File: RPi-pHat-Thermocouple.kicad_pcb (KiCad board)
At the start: 2 copper layers, 65 x 30 mm, 47 parts, among them J1 Screw_Terminal_01x02, J2 RPi_GPIO, J3 Screw_Terminal_01x02, J4 Screw_Terminal_01x02, J5 Screw_Terminal_01x02, J6 Screw_Terminal_01x03, J7 Screw_Terminal_01x04, U1 MCP1754ST, U2 DS18S20, U3 MAX31850K, U4 MAX31850K, U5 MAX31850K, U6 MAX3221CDBR, U7 ADuM1201ARZ

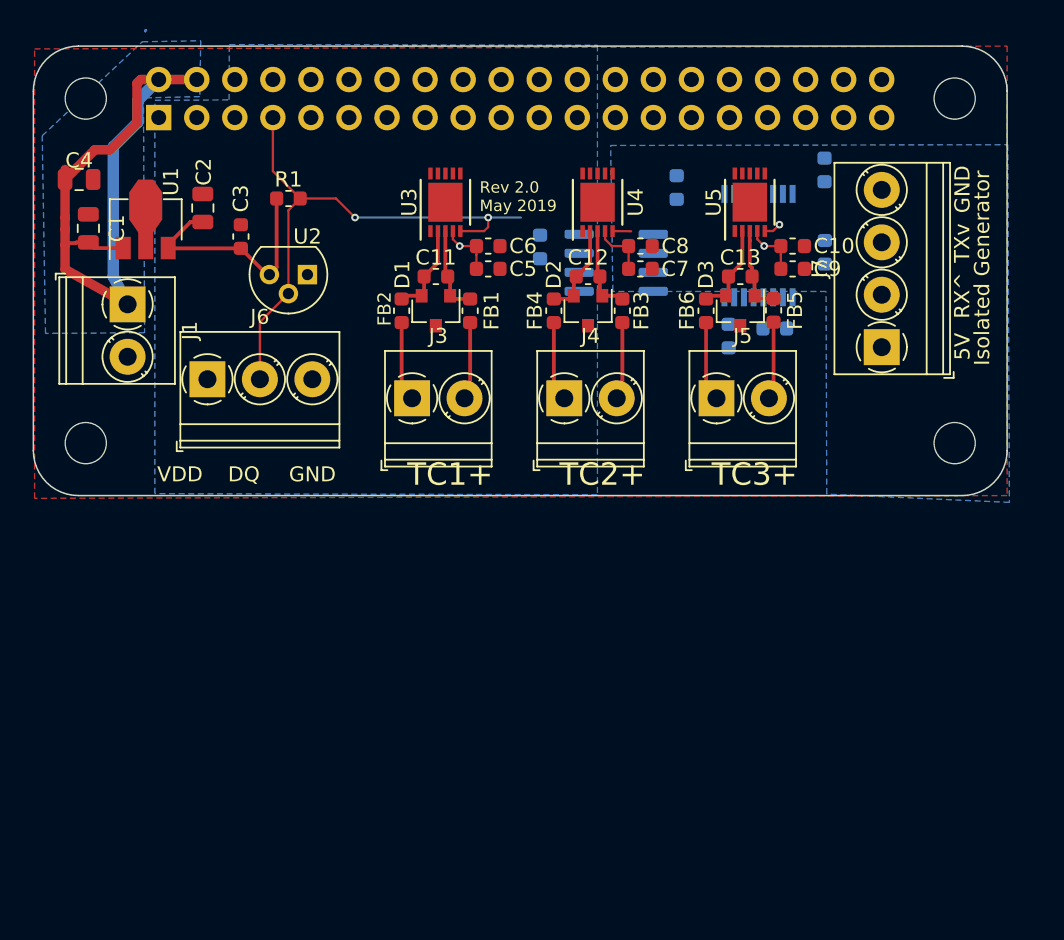
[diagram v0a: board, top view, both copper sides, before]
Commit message: PCB Version 3.0 files
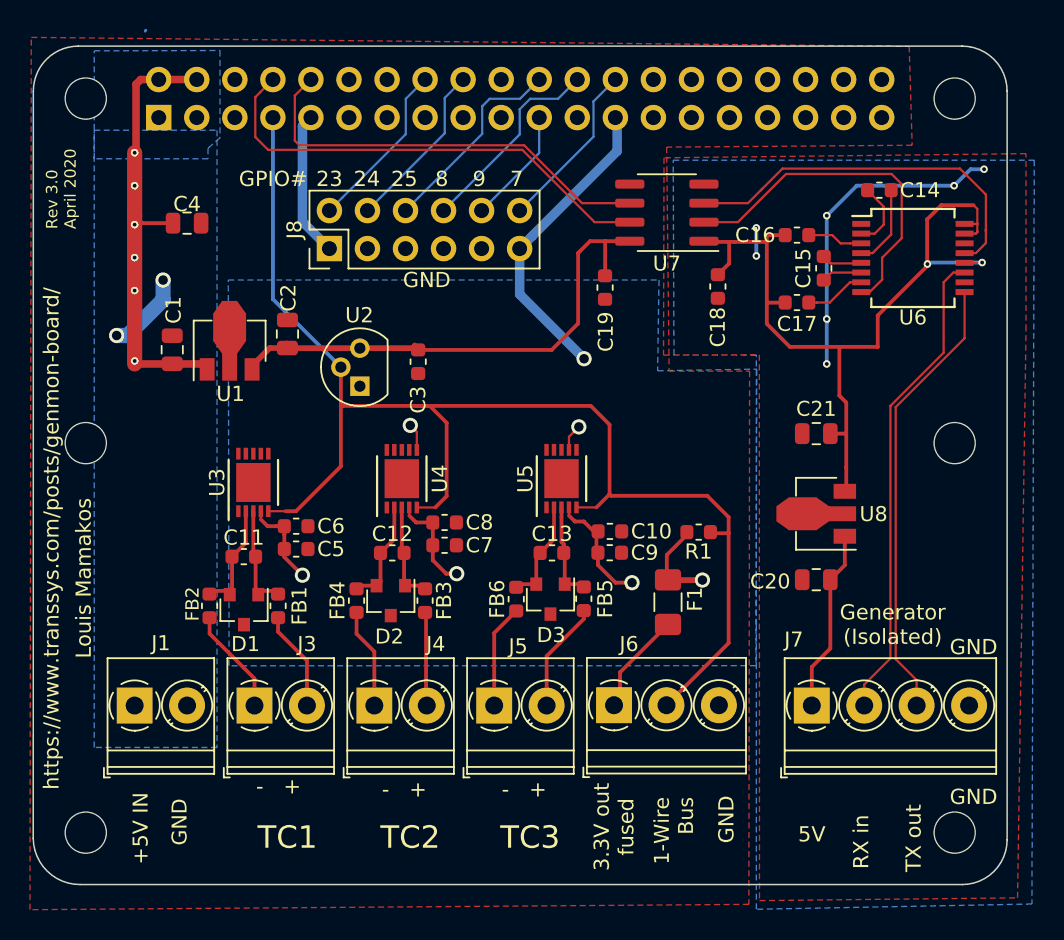
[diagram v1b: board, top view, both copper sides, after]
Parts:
- added C20: 2.2uF, Capacitor_SMD:C_0805_2012Metric, F.Cu at (64.8, 60.1)
- added C21: 2.2uF, Capacitor_SMD:C_0805_2012Metric, F.Cu at (64.8, 50.4)
- added F1: Polyfuse 1206L010/60WR 0.1A, Fuse:Fuse_1206_3216Metric_Pad1.42x1.75mm_HandSolder, F.Cu at (54.9, 61.6)
- added J8: Conn_02x06_Odd_Even, Connector_PinHeader_2.54mm:PinHeader_2x06_P2.54mm_Vertical, F.Cu at (32.3, 38.0)
- added U8: MCP1754ST, Package_TO_SOT_SMD:SOT-89-3, F.Cu at (65.2, 55.7)
- added h5: , RPi_Hat:RPi_Hat_Mounting_Hole, F.Cu at (74.0, 77.0)
- added h6: , RPi_Hat:RPi_Hat_Mounting_Hole, F.Cu at (16.0, 77.0)
- C14, C15, C16, C17, C18, C19, U6: moved to F.Cu
- U3: value MAX31850K -> MAX31850KATB
- U4, U5: value MAX31850K -> MAX31850KATB+T
- U7: value ADuM1201ARZ -> ADuM1201ARZ-RL7; moved to F.Cu
- moved R1 35.3 mm to (56.9, 56.9)
- moved J6 34.8 mm to (51.3, 68.5)
- moved J1 26.8 mm to (19.3, 68.5), turned to 0 degrees
- moved J5 25.3 mm to (43.3, 68.5)
- moved J7 24.4 mm to (64.5, 68.5), turned to 0 degrees
- moved J4 24.1 mm to (35.3, 68.5)
- moved D1 23.7 mm to (26.6, 62.1)
- moved FB2 23.5 mm to (24.3, 61.9)
- moved FB1 23.5 mm to (28.8, 61.9)
- moved D2 23.4 mm to (36.4, 61.5)
- moved FB3 23.4 mm to (38.6, 61.5)
- moved FB4 23.4 mm to (34.1, 61.5)
- moved J3 23.1 mm to (27.3, 68.5)
- moved FB5 23.0 mm to (49.2, 61.4)
- moved FB6 23.0 mm to (44.7, 61.4)
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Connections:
- net /GENGND renamed Net-(C18-Pad2)
- C16 pad 2: /GEN5V -> /GEN3V3
- C17 pad 2: /GEN5V -> /GEN3V3
- C18 pad 1: /GEN5V -> /GEN3V3
- J2 pad 16: Net-(J2-Pad16) -> GPIO23
- J2 pad 18: Net-(J2-Pad18) -> GPIO24
- J2 pad 21: Net-(J2-Pad21) -> /GPIO9
- J2 pad 22: Net-(J2-Pad22) -> GPIO25
- J2 pad 24: Net-(J2-Pad24) -> GPIO8
- J2 pad 26: Net-(J2-Pad26) -> GPIO7
- J6 pad 1: +3.3VA -> Net-(F1-Pad1)
- U6 pad 12: /GEN5V -> /GEN3V3
- U6 pad 15: /GEN5V -> /GEN3V3
- U6 pad 16: /GEN5V -> /GEN3V3
- U7 pad 1: /GEN5V -> /GEN3V3
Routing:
- net /GEN3V3: track 0.00 -> 56.1 mm, vias 0 -> 2
- net /W1: track 39.6 -> 91.2 mm, vias 3 -> 0
- net +3.3VA: track 27.7 -> 66.2 mm, vias 2 -> 6
- net GND: track 0.00 -> 35.7 mm, vias 0 -> 3
- net /TXD: track 0.00 -> 31.7 mm
- net /GENIN: track 0.62 -> 32.1 mm
- net /GENOUT: track 0.00 -> 30.1 mm
- net /RXD: track 0.00 -> 29.3 mm
- net Net-(U6-Pad13): track 0.00 -> 25.8 mm
- net Net-(C18-Pad2): track 0.00 -> 23.7 mm, vias 0 -> 7
- net Net-(U6-Pad8): track 0.00 -> 23.5 mm
- net +5V: track 45.2 -> 31.5 mm, vias 0 -> 6
- net GPIO25: track 0.00 -> 13.6 mm
- net GPIO8: track 0.00 -> 13.5 mm
- net /GEN5V: track 0.00 -> 12.2 mm
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- added copper zone on B.Cu, net /GEN5V
- added copper zone on F.Cu, net Net-(C18-Pad2)
- removed copper zone on B.Cu, net Net-(C18-Pad2)
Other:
- board size 65 x 30 mm -> 65 x 56 mm
- board text added: "+ -"
- board text added: "+3.3V"
- board text added: "+5DC to Raspberry Pi"
- board text added: "+5V IN"
- board text added: "- +"
- board text added: "1-Wire Bus"
- board text added: "23"
- board text added: "24"
- board text added: "25"
- board text added: "3.3V out (fused)"
- board text added: "3.3V out fused"
- board text added: "7"
- board text added: "8"
- board text added: "9"
- board text added: "GND TX RX +5 Isolated Generator Controller Signals"
- board text added: "GPIO#"
- board text added: "Generator (Isolated)"
- board text added: "Generator Controller Isolated +5V"
- board text added: "Generator power supply and RS-232 signals isolated from Raspberry Pi and power supply. Do not interconnect generator ground and power supply with Raspberry Pi power to preserve galvanic isolation from controller and avoid ground loops."
- board text added: "Louis Mamakos"
- board text added: "RX in"
- board text added: "Rev 3.0 April 2020"
- board text added: "TX out"
- board text added: "Thermocouple Hat by Louis Mamakos (based on a design by Mike Lawrence)"
- board text added: "Type K Thermocouple Connections"
- board text added: "^ External DS18B20 temperature sensor connection."
- board text added: "https://www.transsys.com/posts/genmon-board/"
- board text removed: "DQ"
- board text removed: "Isolated Generator"
- board text removed: "RX^"
- board text removed: "Rev 2.0 May 2019"
- board text removed: "TC1+"
- board text removed: "TC2+"
- board text removed: "TC3+"
- board text removed: "TXv"
- board text removed: "Thermocouple pHat by Mike Lawrence"
- board text removed: "VDD"

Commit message: Candidate files for Version 3.1 of the PCB
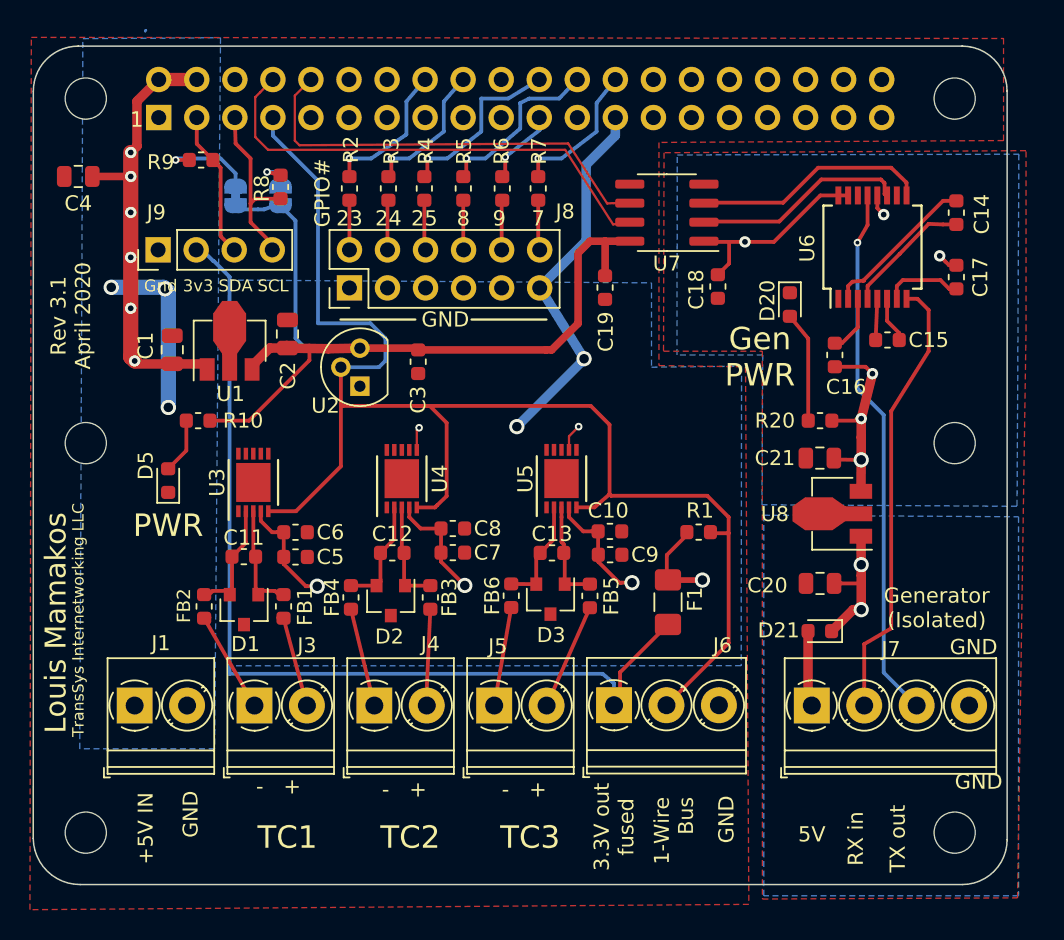
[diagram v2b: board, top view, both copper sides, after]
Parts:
- added D20: ASMT-RF45-AN002, LED_SMD:LED_0603_1608Metric, F.Cu at (63.0, 41.8)
- added D21: NSR20F30NXT5G, Diode_SMD:D_0603_1608Metric, F.Cu at (65.0, 63.5)
- added D5: ASMT-RF45-AN002, LED_SMD:LED_0603_1608Metric, F.Cu at (21.5, 53.5)
- added J9: Conn_01x04_Male, Connector_PinHeader_2.54mm:PinHeader_1x04_P2.54mm_Vertical, F.Cu at (20.8, 38.1)
- added JP1: Jumper_NC_Small, Jumper:SolderJumper-2_P1.3mm_Bridged_RoundedPad1.0x1.5mm, B.Cu at (29.0, 34.5)
- added JP2: Jumper_NC_Small, Jumper:SolderJumper-2_P1.3mm_Bridged_RoundedPad1.0x1.5mm, B.Cu at (26.0, 34.5)
- added R10: 120, Resistor_SMD:R_0603_1608Metric, F.Cu at (23.5, 49.5)
- added R2: 330, Resistor_SMD:R_0603_1608Metric, F.Cu at (33.6, 34.0)
- added R20: 120, Resistor_SMD:R_0603_1608Metric, F.Cu at (65.0, 49.5)
- added R3: 330, Resistor_SMD:R_0603_1608Metric, F.Cu at (36.2, 34.0)
- added R4: 330, Resistor_SMD:R_0603_1608Metric, F.Cu at (38.6, 34.0)
- added R5: 330, Resistor_SMD:R_0603_1608Metric, F.Cu at (41.2, 34.0)
- added R6: 330, Resistor_SMD:R_0603_1608Metric, F.Cu at (43.8, 34.0)
- added R7: 330, Resistor_SMD:R_0603_1608Metric, F.Cu at (46.2, 34.0)
- added R8: 4.7k, Resistor_SMD:R_0603_1608Metric, F.Cu at (29.0, 33.9)
- added R9: 4.7k, Resistor_SMD:R_0603_1608Metric, F.Cu at (23.7, 32.1)
- C14: value 0.047uF -> 0.1uF
- C15, C16, C17: value 0.33uF -> 0.1uF
- U2: value DS18S20 -> DS18B20
- U3: value MAX31850KATB -> MAX31850KATB
- U4, U5: value MAX31850KATB+T -> MAX31850KATB
- U7: value ADuM1201ARZ-RL7 -> ADuM1201AR
- moved C17 10.8 mm to (74.1, 39.9), turned to 90 degrees
- moved C16 8.39 mm to (66.0, 45.1), turned to 270 degrees
- moved C4 7.90 mm to (15.5, 33.2), turned to 180 degrees
- moved C15 6.40 mm to (69.5, 44.1), turned to 0 degrees
- moved C14 5.35 mm to (74.1, 35.6), turned to 270 degrees
- moved J8 2.95 mm to (33.6, 40.6)
- moved U6 2.80 mm to (68.5, 37.9), turned to 90 degrees
- moved C21 1.65 mm to (65.0, 52.0)
- moved U8 1.08 mm to (66.3, 55.7)
- moved C7 0.73 mm to (40.5, 58.3)
- moved C8 0.68 mm to (40.5, 56.7)
- moved C5 0.53 mm to (30.0, 58.6)
- moved FB5 0.45 mm to (49.6, 61.2)
- moved FB4 0.43 mm to (33.7, 61.3)
- moved FB3 0.41 mm to (39.0, 61.3)
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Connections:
- net /GEN3V3 renamed +3V3
- net /RXD renamed Net-(J2-Pad10)
- net Net-(C18-Pad2) renamed GNDD
- net Net-(F1-Pad1) renamed /3V3FUSED
- J2 pad 3: Net-(J2-Pad3) -> /SDA
- J2 pad 5: Net-(J2-Pad5) -> /SCL
- J7 pad 1: /GEN5V -> Net-(D21-Pad2)
- J8 pad 10: /GPIO9 -> Net-(J8-Pad10)
- J8 pad 12: GPIO7 -> Net-(J8-Pad12)
- J8 pad 2: GPIO23 -> Net-(J8-Pad2)
- J8 pad 4: GPIO24 -> Net-(J8-Pad4)
- J8 pad 6: GPIO25 -> Net-(J8-Pad6)
- J8 pad 8: GPIO8 -> Net-(J8-Pad8)
- U6 pad 11: /GENIN -> /GEN-OUT-TTL
- U6 pad 13: Net-(U6-Pad13) -> /GENOUT
- U6 pad 8: Net-(U6-Pad8) -> /GENIN
- U6 pad 9: /GENOUT -> /GEN-IN-TTL
- U7 pad 2: Net-(U6-Pad8) -> /GEN-OUT-TTL
- U7 pad 3: Net-(U6-Pad13) -> /GEN-IN-TTL
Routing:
- net /3V3FUSED: track 6.72 -> 63.3 mm
- net +3.3VA: track 66.2 -> 95.3 mm
- net Net-(U6-Pad13): track 25.8 -> 0.00 mm
- net +3V3: track 56.1 -> 30.9 mm, vias 2 -> 6
- net GNDD: track 23.7 -> 0.00 mm, vias 7 -> 0
- net Net-(U6-Pad8): track 23.5 -> 0.00 mm
- net /GEN-IN-TTL: track 0.00 -> 16.7 mm
- net /GEN-OUT-TTL: track 0.00 -> 14.3 mm
- net /SCL: track 0.00 -> 12.0 mm
- net /SDA: track 0.00 -> 9.86 mm
- net Net-(D20-Pad2): track 0.00 -> 7.40 mm
- net Net-(JP2-Pad1): track 0.00 -> 6.37 mm, vias 0 -> 1
- net Net-(C14-Pad1): track 4.49 -> 10.5 mm
- net /GENOUT: track 30.1 -> 35.9 mm, vias 0 -> 1
- net /W1: track 91.2 -> 96.9 mm
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- added copper zone on B.Cu, net +3V3
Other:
- board text added: "1"
- board text added: "3v3"
- board text added: "Cut links to disable I2C pull-ups"
- board text added: "Do not connect external power if Raspberry Pi is USB Powered"
- board text added: "GND TX RX +5 Isolated Generator Signals"
- board text added: "Gen PWR"
- board text added: "Generator Isolated +3.3V"
- board text added: "Gnd"
- board text added: "I2C expansion"
- board text added: "PWR"
- board text added: "Rev 3.1 April 2020"
- board text added: "SCL"
- board text added: "SCL PU"
- board text added: "SCL SDA 3v3 GND"
- board text added: "SDA"
- board text added: "SDA PU"
- board text added: "Thermocouple Hat by Louis Mamakos"
- board text added: "TransSys Internetworking LLC"
- board text added: "WARNING"
- board text added: "ext +5VDC"
- board text removed: "GND TX RX +5 Isolated Generator Controller Signals"
- board text removed: "Generator power supply and RS-232 signals isolated from Raspberry Pi and power supply. Do not interconnect generator ground and power supply with Raspberry Pi power to preserve galvanic isolation from controller and avoid ground loops."
- board text removed: "Rev 3.0 April 2020"
- board text removed: "Thermocouple Hat by Louis Mamakos (based on a design by Mike Lawrence)"
